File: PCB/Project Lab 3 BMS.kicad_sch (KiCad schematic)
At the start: 37 parts, among them J1 Conn_01x04, J2 Screw_Terminal_01x02, Q1 CSD17571Q2T, Q2 CSD17571Q2T, U1 BQ76920PW, U2 ESP32-WROOM-32, U3 LD1086V33-DG

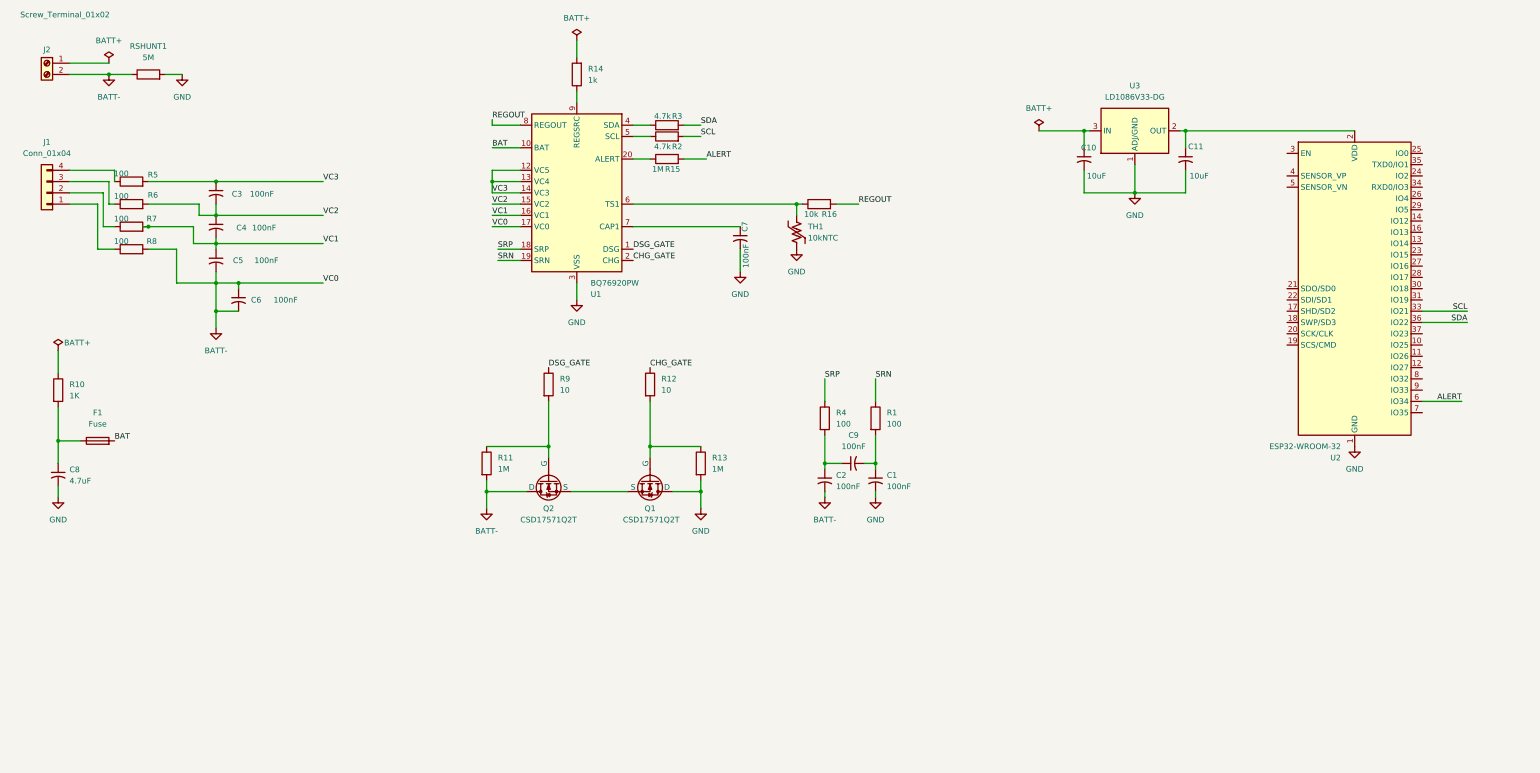
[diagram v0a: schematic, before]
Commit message: update
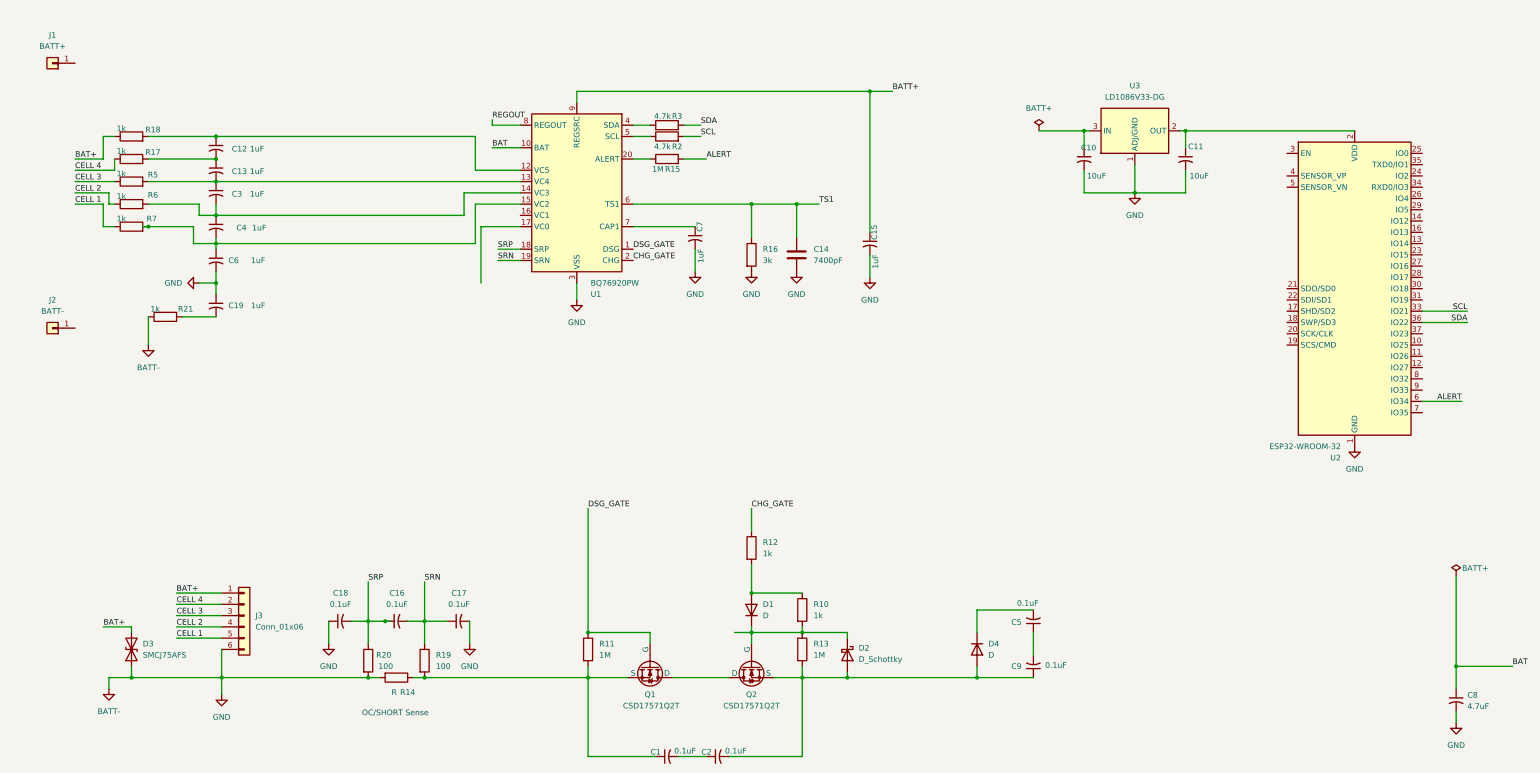
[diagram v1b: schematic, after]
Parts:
- removed F1: Fuse, symbol Device:Fuse
- removed J1: Conn_01x04, symbol Connector_Generic:Conn_01x04
- removed J2: Screw_Terminal_01x02, symbol Connector:Screw_Terminal_01x02
- removed R1, R4, R8: 100, symbol Device:R
- removed R9: 10, symbol Device:R
- removed RSHUNT1: 5M, symbol Device:R
- removed TH1: 10kNTC, symbol Device:Thermistor_US
- added C12, C13, C15, C19: 1uF, symbol Device:C_Small_US
- added C14: 7400pF, symbol Device:C
- added C16, C17, C18: 0.1uF, symbol Device:C_Small_US
- added D1, D4: D, symbol Device:D
- added D2: D_Schottky, symbol Device:D_Schottky
- added D3: SMCJ75AFS, symbol Device:D_TVS
- added J1: BATT+, symbol Connector_Generic:Conn_01x01
- added J2: BATT-, symbol Connector_Generic:Conn_01x01
- added J3: Conn_01x06, symbol Connector_Generic:Conn_01x06
- added R17, R18, R21: 1k, symbol Device:R
- added R19, R20: 100, symbol Device:R
- C1, C2, C5, C9: value 100nF -> 0.1uF
- C3, C4, C6, C7: value 100nF -> 1uF
- R10: value 1K -> 1k
- R12: value 10 -> 1k
- R14: value 1k -> R
- R16: value 10k -> 3k
- R5, R6, R7: value 100 -> 1k
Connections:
- net BAT: now also C8.1
- net BATT-: now also C10.2, C11.2, C7.2, C8.2, R14.2, R16.2, U1.3 (VSS), U2.1 (GND), U2.15 (GND), U2.38 (GND), U2.39 (GND), U3.1 (ADJ/GND), C14.2, C15.2, C17.2, C18.1, C19.1, D3.1 (A1), J3.6 (Pin_6), R20.2, R21.1; no longer C2.2, C5.2, C6.1, Q2.1 (D), R11.2, U1.17 (VC0)
- net DSG_GATE: now also Q1.2 (G), R11.1
- net REGOUT: no longer R16.2
- net SRN: now also C16.2, C17.1, R19.1
- net SRP: now also C16.1, C18.2, R20.1
- net at C9.1: now also C2.2, Q2.3 (S), R13.2, D2.2 (A), D4.2 (A); no longer C2.1
- net at C1.1: now also Q1.3 (S), R11.2, R14.1, R19.2; no longer C9.2
- net TS1: now reaches R16.1, U1.6 (TS1)
- net TS1: now also C14.1
- net at Q2.2 (G): now also R10.2, R13.1, D1.1 (K), D2.1 (K); no longer R11.1
- net CELL 3: now reaches R5.1
- net CELL 3: now also J3.3 (Pin_3)
- net CELL 2: now reaches R6.1
- net CELL 2: now also J3.4 (Pin_4)
- net at R7.1: no longer names the net of R7.1
- net at R7.1: now also J3.5 (Pin_5)
- net at R10.1: now also R12.2, D1.2 (A)
- net BATT+: now reaches U1.9 (REGSRC)
- net BATT+: now also C15.1; no longer R14.1
- removed net GND: C1.2, C10.2, C11.2, C7.2, C8.2, Q1.1 (D), R13.2, U1.3 (VSS), U2.1 (GND), U2.15 (GND), U2.38 (GND), U2.39 (GND), U3.1 (ADJ/GND)
- net VC1: no longer names the net of C4.2, R7.2
- net VC1: now also C6.1, U1.15 (VC2); no longer C5.1, U1.16 (VC1)
- net VC2: no longer names the net of C3.2, C4.1, R6.2
- net VC2: now also U1.14 (VC3); no longer U1.15 (VC2)
- net VC3: no longer names the net of C3.1, R5.2, U1.13 (VC4)
- net VC3: now also C13.2; no longer U1.12 (VC5), U1.14 (VC3)
- new net: C19.2, R21.2
- new net: C12.1, R18.2, U1.12 (VC5)
- new net: C1.2, C2.1
- new net: C5.2, D4.1 (K)
- new net: C5.1, C9.2
- new net: C12.2, C13.1, R17.2
- new net: Q1.1 (D), Q2.1 (D)
- new net BAT+: D3.2 (A2), J3.1 (Pin_1), R18.1
- new net CELL 4: J3.2 (Pin_2), R17.1
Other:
- note added: "OC/SHORT Sense"
- moved on the sheet: C6, C7, C8, Q1, Q2, R11, R13
